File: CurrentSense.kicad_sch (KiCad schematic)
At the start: 10 parts, among them J2 1935161, J4 SJ2-35813B-SMT-TR

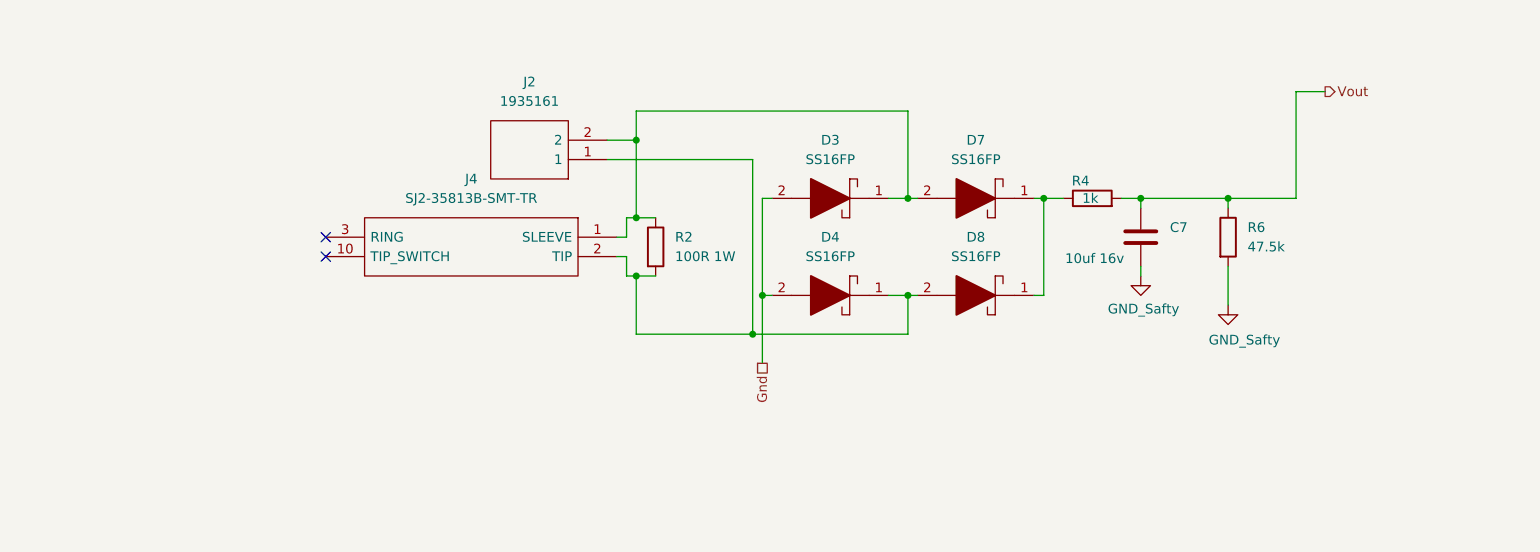
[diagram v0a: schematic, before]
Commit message: progress
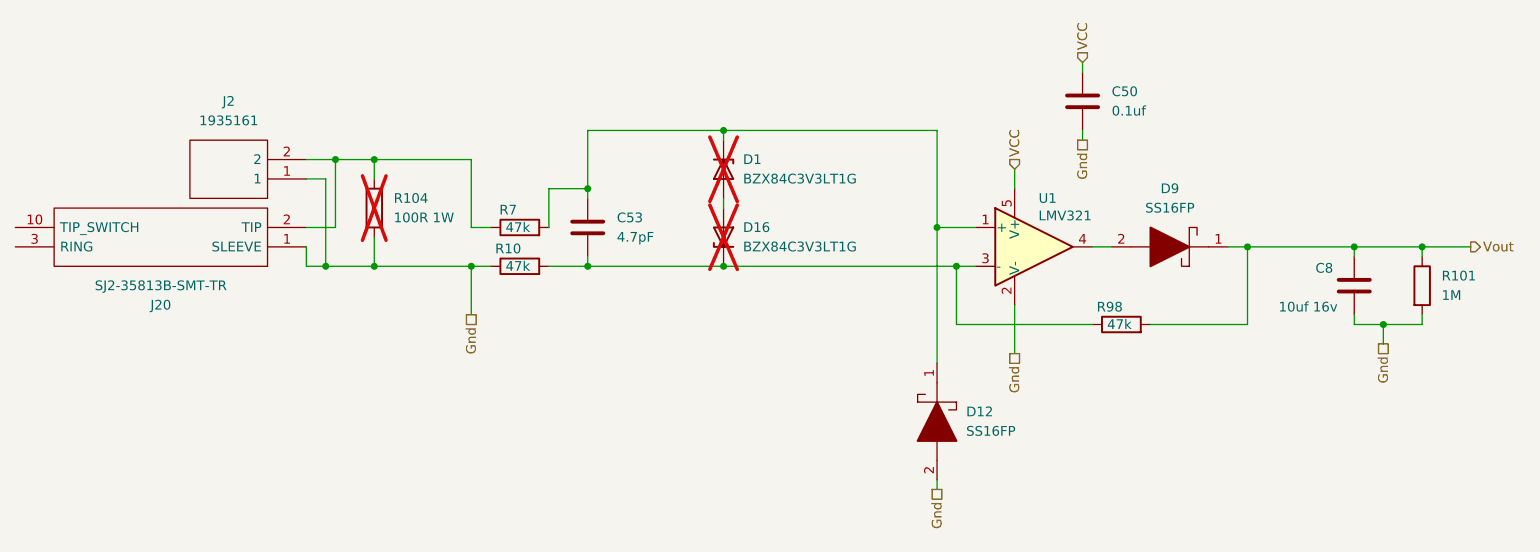
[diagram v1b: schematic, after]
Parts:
- removed C7: 10uf 16v, Capacitor_SMD:C_0805_2012Metric, symbol Device:C
- removed D3, D4, D7, D8: SS16FP, SamacSys_Parts:SS12FP, symbol SamacSys_Parts:SS16FP
- removed J4: SJ2-35813B-SMT-TR, SamacSys_Parts:SJ235813BSMTTR, symbol SamacSys_Parts:SJ2-35813B-SMT-TR
- removed R2: 100R 1W, Resistor_SMD:R_2512_6332Metric, symbol Device:R
- removed R4: 1k, Resistor_SMD:R_0402_1005Metric, symbol Device:R
- removed R6: 47.5k, Resistor_SMD:R_0402_1005Metric, symbol Device:R
- added C50: 0.1uf, Capacitor_SMD:C_0402_1005Metric, symbol Device:C
- added C53: 4.7pF, Capacitor_SMD:C_0402_1005Metric, symbol Device:C
- added C8: 10uf 16v, Capacitor_SMD:C_0805_2012Metric, symbol Device:C
- added D1, D16: BZX84C3V3LT1G, Package_TO_SOT_SMD:SOT-23, symbol Diode:BZX84Cxx
- added D12, D9: SS16FP, SamacSys_Parts:SS12FP, symbol SamacSys_Parts:SS16FP
- added J20: SJ2-35813B-SMT-TR, SamacSys_Parts:SJ235813BSMTTR, symbol SamacSys_Parts:SJ2-35813B-SMT-TR
- added R10, R7, R98: 47k, Resistor_SMD:R_0402_1005Metric, symbol Device:R
- added R101: 1M, Resistor_SMD:R_0402_1005Metric, symbol Device:R
- added R104: 100R 1W, Resistor_SMD:R_2512_6332Metric, symbol Device:R
- added U1: LMV321, Package_TO_SOT_SMD:SOT-353_SC-70-5, symbol Amplifier_Operational:LMV321
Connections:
- net Gnd: now also J2.1, C50.2, C8.2, D12.2, J20.1 (SLEEVE), R10.1, R101.2, R104.2, U1.2 (V-)
- net Vout: now also C8.1, D9.1, R101.1, R98.2
- net at J2.2: now also J20.2 (TIP), R104.1, R7.1
- new net: D1.1 (A), D16.1 (A)
- new net: C53.2, D16.3 (K), R10.2, R98.1, U1.3 (-)
- new net: C53.1, D1.3 (K), D12.1, R7.2, U1.1 (+)
- new net: D9.2, U1.4
- new net VCC: C50.1, U1.5 (V+)
- no-connect marks 2 -> 0
